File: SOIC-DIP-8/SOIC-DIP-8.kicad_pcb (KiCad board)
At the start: 2 copper layers, 2 parts, among them J1 Conn_02x04_Counter_Clockwise, J2 Conn_02x04_Counter_Clockwise

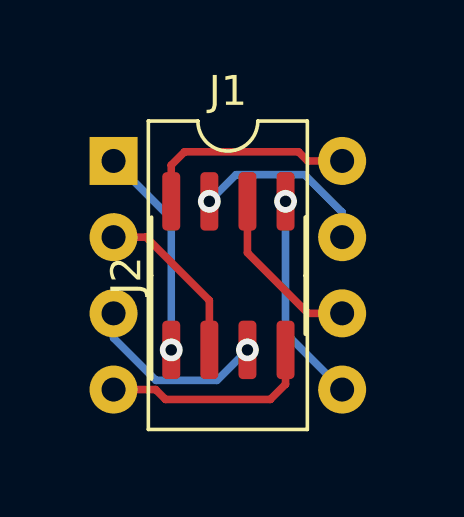
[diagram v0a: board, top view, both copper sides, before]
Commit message: Boards sent to be built.
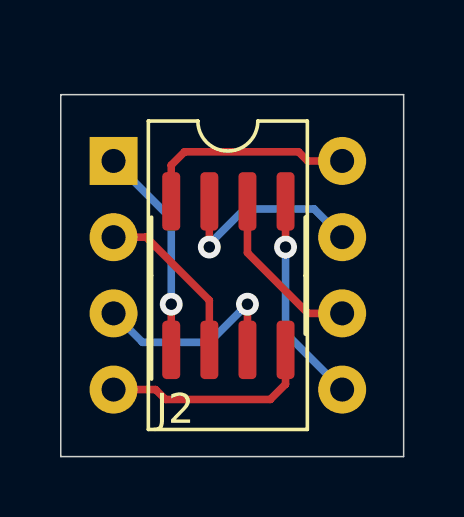
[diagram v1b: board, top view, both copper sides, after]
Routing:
- net /Pin7: track 6.14 -> 6.92 mm
- net /Pin3: track 6.29 -> 6.91 mm
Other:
- board outline added: 11.4 x 12.1 mm
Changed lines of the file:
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@@
   (general
     (thickness 1.6)
-    (drawings 0)
-    (tracks 33)
+    (drawings 6)
+    (tracks 37)
     (zones 0)
     (modules 2)
@@
     (solder_mask_min_width 0.25)
     (aux_axis_origin 0 0)
-    (visible_elements FFFFFF7F)
+    (grid_origin 130.81 79.375)
+    (visible_elements 7FFFFFFF)
     (pcbplotparams
       (layerselection 0x010fc_ffffffff)
@@
       (outputformat 1)
       (mirror false)
-      (drillshape 1)
+      (drillshape 0)
       (scaleselection 1)
       (outputdirectory ""))
@@
     (descr "8-lead though-hole mounted DIP package, row spacing 7.62 mm (300 mils)")
     (tags "THT DIP DIL PDIP 2.54mm 7.62mm 300mil")
-    (fp_text reference J1 (at 3.81 -2.33) (layer F.SilkS)
+    (fp_text reference J1 (at 2.049999 0.012499) (layer B.SilkS)
       (effects (font (size 1 1) (thickness 0.15)))
     )
@@
     (tags "SOIC SO")
     (attr smd)
-    (fp_text reference J2 (at 0 -3.4 90) (layer F.SilkS)
+    (fp_text reference J2 (at -4.445 -1.778 180) (layer F.SilkS)
       (effects (font (size 1 1) (thickness 0.15)))
     )
@@
     )
   )
+  (dimension 12.065 (width 0.15) (layer Dwgs.User)
+    (gr_text "0.4750 in" (at 127.605 73.3425 90) (layer Dwgs.User)
+      (effects (font (size 1 1) (thickness 0.15)))
+    )
+    (feature1 (pts (xy 130.81 67.31) (xy 128.318579 67.31)))
+    (feature2 (pts (xy 130.81 79.375) (xy 128.318579 79.375)))
+    (crossbar (pts (xy 128.905 79.375) (xy 128.905 67.31)))
+    (arrow1a (pts (xy 128.905 67.31) (xy 129.491421 68.436504)))
+    (arrow1b (pts (xy 128.905 67.31) (xy 128.318579 68.436504)))
+    (arrow2a (pts (xy 128.905 79.375) (xy 129.491421 78.248496)))
+    (arrow2b (pts (xy 128.905 79.375) (xy 128.318579 78.248496)))
+  )
+  (dimension 11.43 (width 0.15) (layer Dwgs.User)
+    (gr_text "0.4500 in" (at 136.525 64.105) (layer Dwgs.User)
+      (effects (font (size 1 1) (thickness 0.15)))
+    )
+    (feature1 (pts (xy 142.24 67.31) (xy 142.24 64.818579)))
+    (feature2 (pts (xy 130.81 67.31) (xy 130.81 64.818579)))
+    (crossbar (pts (xy 130.81 65.405) (xy 142.24 65.405)))
+    (arrow1a (pts (xy 142.24 65.405) (xy 141.113496 65.991421)))
+    (arrow1b (pts (xy 142.24 65.405) (xy 141.113496 64.818579)))
+    (arrow2a (pts (xy 130.81 65.405) (xy 131.936504 65.991421)))
+    (arrow2b (pts (xy 130.81 65.405) (xy 131.936504 64.818579)))
+  )
+  (gr_line (start 142.24 79.375) (end 130.81 79.375) (layer Edge.Cuts) (width 0.05))
+  (gr_line (start 142.24 67.31) (end 142.24 79.375) (layer Edge.Cuts) (width 0.05))
+  (gr_line (start 130.81 67.31) (end 142.24 67.31) (layer Edge.Cuts) (width 0.05))
+  (gr_line (start 130.81 79.375) (end 130.81 67.31) (layer Edge.Cuts) (width 0.05))
   (segment (start 139.885 69.215) (end 140.190001 69.520001) (width 0.254) (layer B.Cu) (net 1))
   (segment (start 139.040002 69.520001) (end 140.190001 69.520001) (width 0.254) (layer F.Cu) (net 1))
@@
   (segment (start 133.972501 77.140001) (end 132.570001 77.140001) (width 0.254) (layer F.Cu) (net 2))
   (segment (start 134.3025 77.47) (end 133.972501 77.140001) (width 0.254) (layer F.Cu) (net 2))
-  (via (at 135.763 70.866) (size 0.762) (drill 0.381) (layers F.Cu B.Cu) (net 3))
-  (via (at 138.303 70.866) (size 0.762) (drill 0.381) (layers F.Cu B.Cu) (net 6))
-  (segment (start 138.938 69.977) (end 140.190001 71.229001) (width 0.254) (layer B.Cu) (net 3))
-  (segment (start 140.190001 71.229001) (end 140.190001 72.060001) (width 0.254) (layer B.Cu) (net 3))
-  (segment (start 135.763 70.866) (end 136.652 69.977) (width 0.254) (layer B.Cu) (net 3))
-  (segment (start 136.652 69.977) (end 138.938 69.977) (width 0.254) (layer B.Cu) (net 3))
-  (via (at 137.033 75.819) (size 0.762) (drill 0.381) (layers F.Cu B.Cu) (net 4))
-  (segment (start 132.570001 75.420001) (end 132.570001 74.600001) (width 0.254) (layer B.Cu) (net 4))
-  (segment (start 133.985 76.835) (end 132.570001 75.420001) (width 0.254) (layer B.Cu) (net 4))
-  (segment (start 137.033 75.819) (end 136.017 76.835) (width 0.254) (layer B.Cu) (net 4))
-  (segment (start 136.017 76.835) (end 133.985 76.835) (width 0.254) (layer B.Cu) (net 4))
+  (via (at 135.763 72.39) (size 0.762) (drill 0.381) (layers F.Cu B.Cu) (net 3))
+  (segment (start 135.763 70.8675) (end 135.763 72.39) (width 0.254) (layer F.Cu) (net 3))
+  (segment (start 140.190001 72.054501) (end 140.190001 72.060001) (width 0.254) (layer B.Cu) (net 3))
+  (segment (start 139.2555 71.12) (end 140.190001 72.054501) (width 0.254) (layer B.Cu) (net 3))
+  (segment (start 136.93775 71.12) (end 139.2555 71.12) (width 0.254) (layer B.Cu) (net 3))
+  (segment (start 135.763 72.39) (end 135.763 72.29475) (width 0.254) (layer B.Cu) (net 3))
+  (segment (start 135.763 72.29475) (end 136.93775 71.12) (width 0.254) (layer B.Cu) (net 3))
+  (segment (start 137.033 75.8175) (end 137.033 74.295) (width 0.254) (layer F.Cu) (net 4))
+  (via (at 137.033 74.295) (size 0.762) (drill 0.381) (layers F.Cu B.Cu) (net 4))
+  (segment (start 135.763 75.565) (end 137.033 74.295) (width 0.254) (layer B.Cu) (net 4))
+  (segment (start 132.570001 74.600001) (end 133.535 75.565) (width 0.254) (layer B.Cu) (net 4))
+  (segment (start 133.535 75.565) (end 135.763 75.565) (width 0.254) (layer B.Cu) (net 4))
   (segment (start 135.763 74.168) (end 135.763 75.8175) (width 0.254) (layer F.Cu) (net 5))
   (segment (start 132.570001 72.060001) (end 133.655001 72.060001) (width 0.254) (layer F.Cu) (net 5))
   (segment (start 133.655001 72.060001) (end 135.763 74.168) (width 0.254) (layer F.Cu) (net 5))
   (segment (start 138.303 75.253) (end 140.190001 77.140001) (width 0.254) (layer B.Cu) (net 6))
-  (segment (start 138.303 70.866) (end 138.303 75.253) (width 0.254) (layer B.Cu) (net 6))
-  (via (at 134.493 75.819) (size 0.762) (drill 0.381) (layers F.Cu B.Cu) (net 7))
+  (via (at 138.303 72.39) (size 0.762) (drill 0.381) (layers F.Cu B.Cu) (net 6))
+  (segment (start 138.303 72.39) (end 138.303 75.253) (width 0.254) (layer B.Cu) (net 6))
+  (segment (start 138.303 70.8675) (end 138.303 72.39) (width 0.254) (layer F.Cu) (net 6))
   (segment (start 134.493 71.443) (end 132.570001 69.520001) (width 0.254) (layer B.Cu) (net 7))
-  (segment (start 134.493 75.819) (end 134.493 71.443) (width 0.254) (layer B.Cu) (net 7))
+  (via (at 134.493 74.295) (size 0.762) (drill 0.381) (layers F.Cu B.Cu) (net 7))
+  (segment (start 134.493 74.295) (end 134.493 71.443) (width 0.254) (layer B.Cu) (net 7))
+  (segment (start 134.493 75.8175) (end 134.493 74.295) (width 0.254) (layer F.Cu) (net 7))
   (segment (start 139.052501 74.600001) (end 140.190001 74.600001) (width 0.254) (layer F.Cu) (net 8))
   (segment (start 137.033 70.8675) (end 137.033 72.5805) (width 0.254) (layer F.Cu) (net 8))
